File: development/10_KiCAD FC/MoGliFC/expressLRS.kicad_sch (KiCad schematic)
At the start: 46 parts, among them SW1 SKTAAAE010, U1 ESP32-PICO-D4, U3 ANT3216LL00R2400A

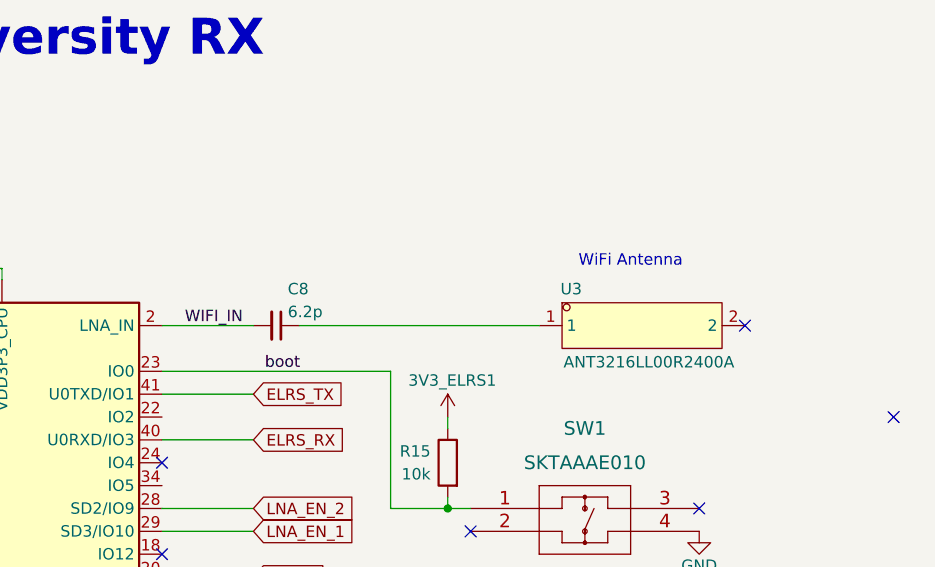
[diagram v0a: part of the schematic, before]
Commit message: Update expressLRS.kicad_sch
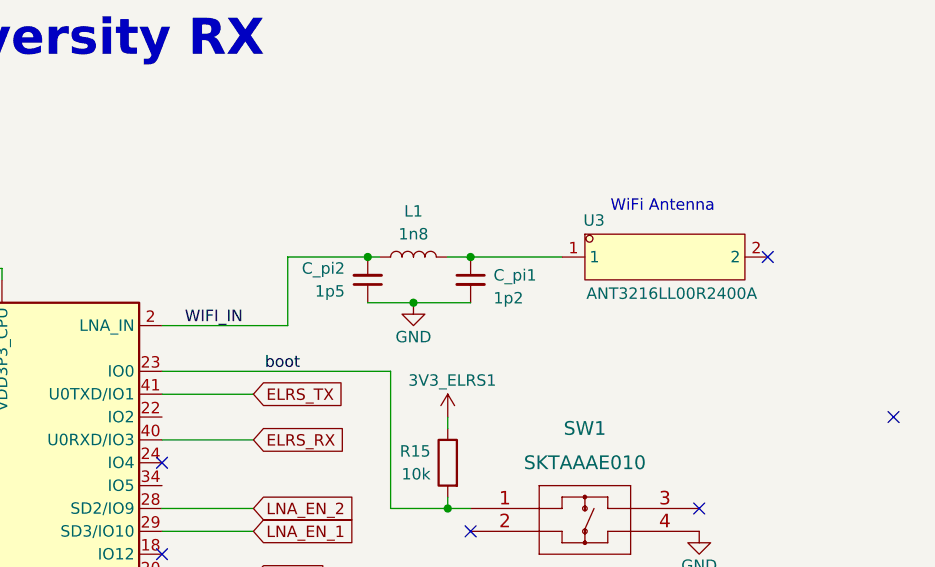
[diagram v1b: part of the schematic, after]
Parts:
- removed C8: 6.2p, Capacitor_SMD:C_0603_1608Metric, symbol Device:C_Small
- added C_pi1: 1p2, Capacitor_SMD:C_0603_1608Metric, symbol Device:C_Small
- added C_pi2: 1p5, Capacitor_SMD:C_0603_1608Metric, symbol Device:C_Small
- added L1: 1n8, symbol Device:L
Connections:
- net GND: now also C_pi1.2, C_pi2.1
- net WIFI_IN: now also C_pi2.2, L1.1
- net at U3.1: now also C_pi1.1, L1.2
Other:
- moved on the sheet: U3
